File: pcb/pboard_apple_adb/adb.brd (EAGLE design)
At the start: 56 x 65 mm, 24 parts, among them IC3 STM32F042F4, SW1 324_SW, SW2 324_SW, SW4 324_SW

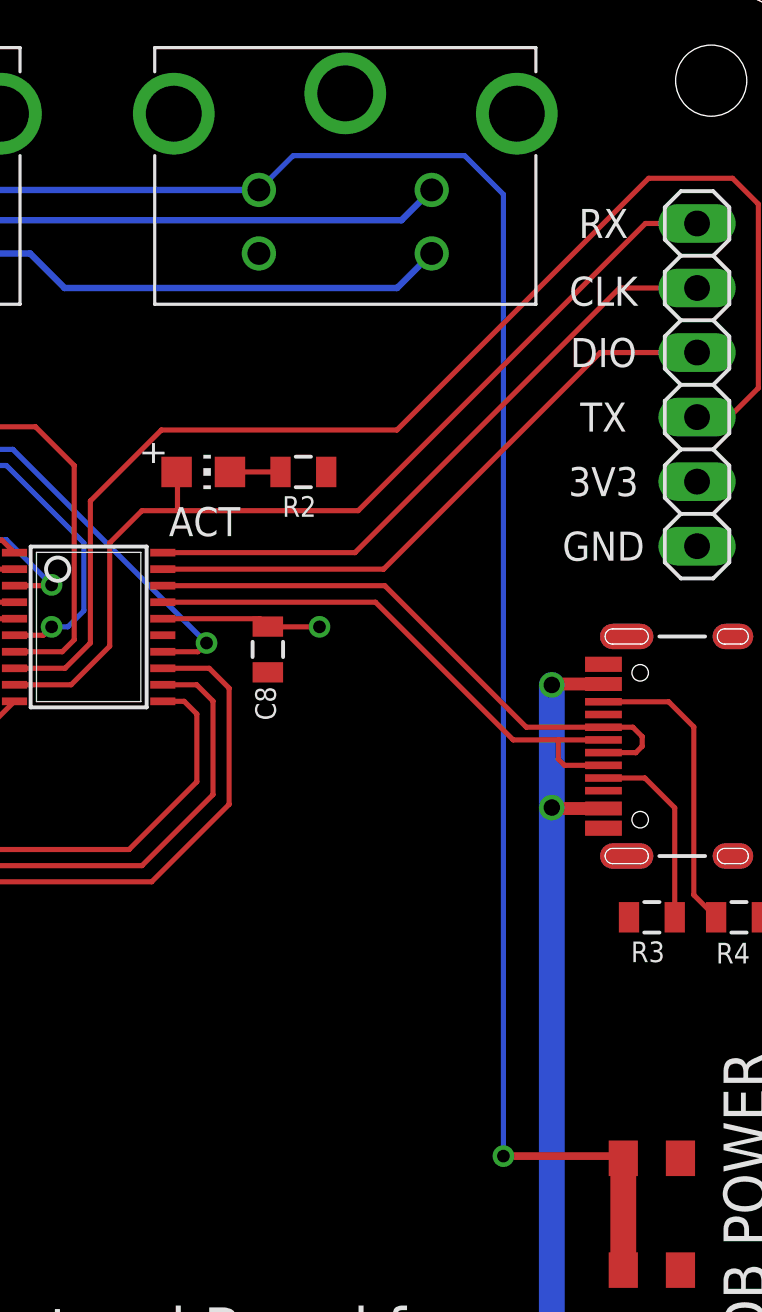
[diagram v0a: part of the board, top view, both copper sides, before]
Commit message: finishing touches for new boards
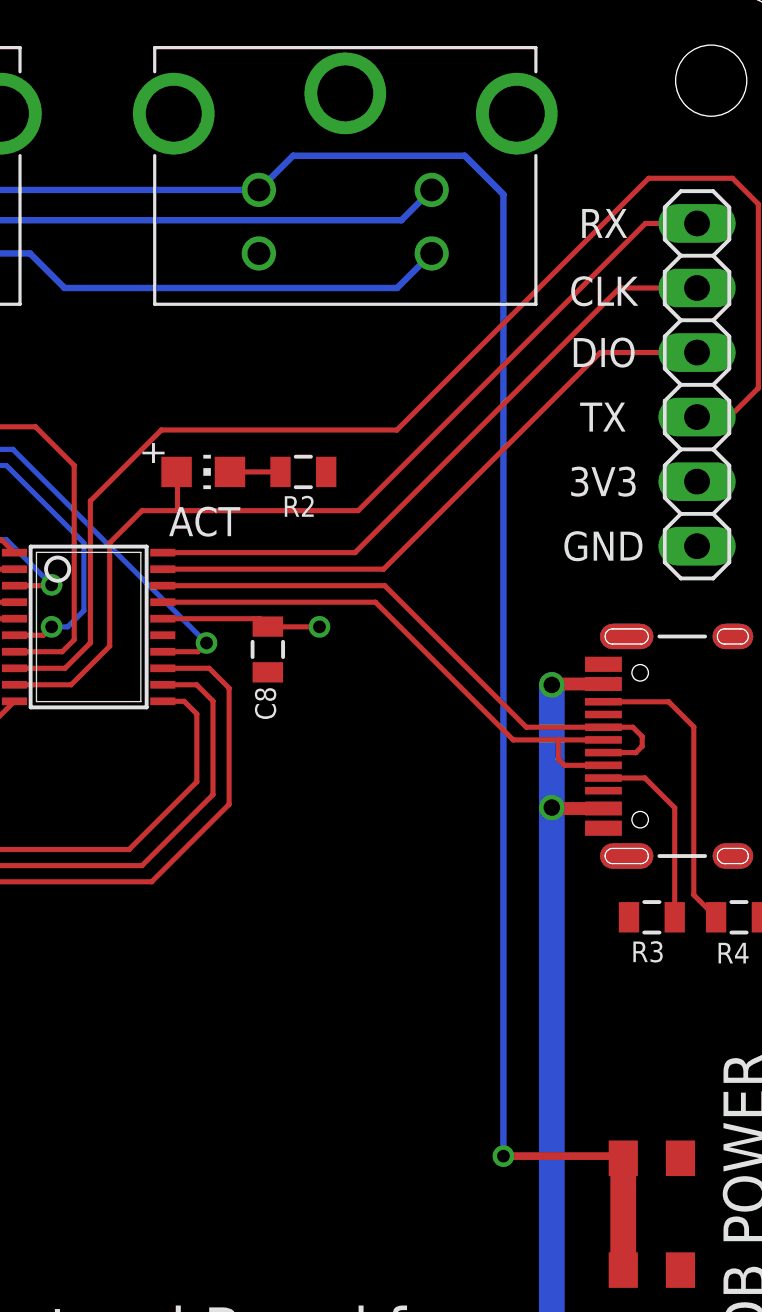
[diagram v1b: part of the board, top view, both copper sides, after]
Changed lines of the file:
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@@
 <wire x1="16.51" y1="49.022" x2="16.51" y2="50.419" width="0.2032" layer="16"/>
 <wire x1="19.177" y1="46.355" x2="16.51" y2="49.022" width="0.2032" layer="16"/>
-<wire x1="34.7" y1="57.2" x2="36.047" y2="58.547" width="0.2032" layer="16"/>
-<wire x1="42.799" y1="58.547" x2="44.323" y2="57.023" width="0.2032" layer="16"/>
-<wire x1="44.323" y1="57.023" x2="44.323" y2="19.177" width="0.2032" layer="16"/>
+<wire x1="34.7" y1="57.2" x2="36.047" y2="58.547" width="0.254" layer="16"/>
+<wire x1="42.799" y1="58.547" x2="44.323" y2="57.023" width="0.254" layer="16"/>
+<wire x1="44.323" y1="57.023" x2="44.323" y2="19.177" width="0.254" layer="16"/>
 <via x="44.323" y="19.177" extent="1-16" drill="0.5"/>
-<wire x1="36.047" y1="58.547" x2="42.799" y2="58.547" width="0.2032" layer="16"/>
+<wire x1="36.047" y1="58.547" x2="42.799" y2="58.547" width="0.254" layer="16"/>
 <wire x1="49.04" y1="19.091" x2="49.04" y2="14.691" width="1.016" layer="1"/>
 <wire x1="49.04" y1="19.091" x2="48.954" y2="19.177" width="0.3048" layer="1"/>
